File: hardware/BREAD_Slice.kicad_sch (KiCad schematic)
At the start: 27 parts, among them J1 I2C_01x04, J2 Conn_01x10_Female, J3 Screw_Terminal_01x02, J4 Screw_Terminal_01x02, J5 Screw_Terminal_01x02, J6 Screw_Terminal_01x02, J7 Screw_Terminal_01x02, J8 Screw_Terminal_01x02, Q1 TIP120, Q2 TIP120, Q3 TIP120, Q4 TIP120

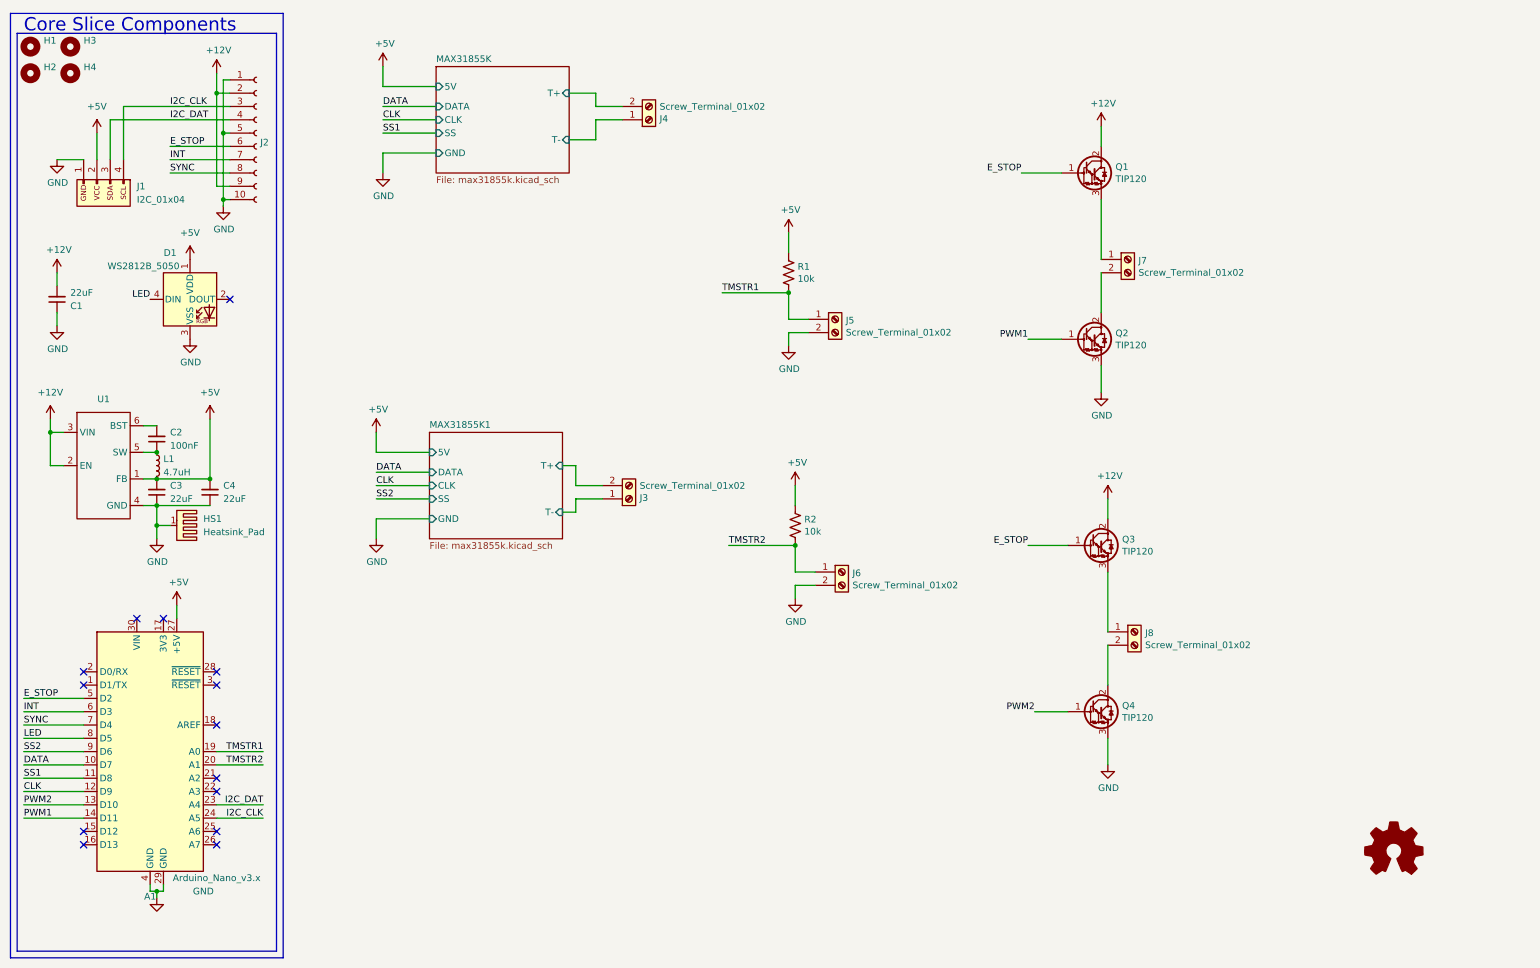
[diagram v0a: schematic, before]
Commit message: JLCPCB order rev-A
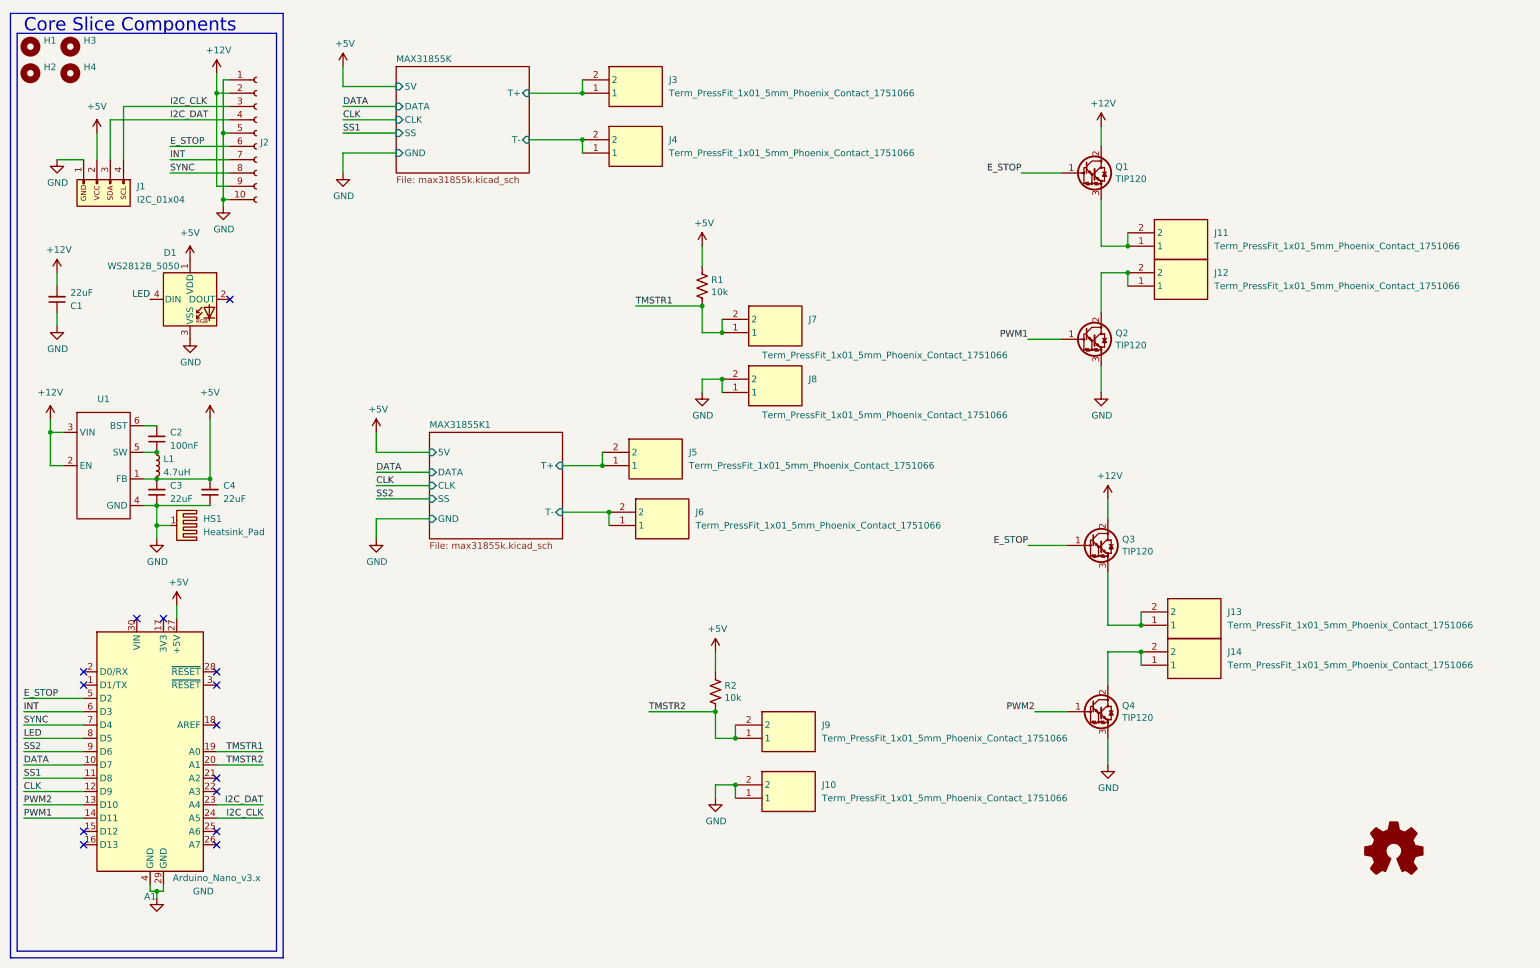
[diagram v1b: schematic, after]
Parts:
- removed J3, J4, J5, J6: Screw_Terminal_01x02, TerminalBlock_Phoenix:TerminalBlock_Phoenix_MPT-0,5-2-2.54_1x02_P2.54mm_Horizontal, symbol Connector:Screw_Terminal_01x02
- removed J7, J8: Screw_Terminal_01x02, TerminalBlock_Phoenix:TerminalBlock_Phoenix_MKDS-1,5-2_1x02_P5.00mm_Horizontal, symbol Connector:Screw_Terminal_01x02
- added J10, J11, J12, J13, J14, J3, J4, J5, J6, J7, J8, J9: Term_PressFit_1x01_5mm_Phoenix_Contact_1751066, 1751066, symbol kml-custom:Term_PressFit_1x01_5mm_Phoenix_Contact_1751066
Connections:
- net GND: now also J10.1, J10.2, J8.1, J8.2
- net MAX31855K/T+: now also J3.1, J3.2
- net MAX31855K/T-: now also J4.1, J4.2
- net MAX31855K1/T+: now also J5.1, J5.2
- net MAX31855K1/T-: now also J6.1, J6.2
- net TMSTR1: now also J7.1, J7.2
- net TMSTR2: now also J9.1, J9.2
- net at Q1.3 (E): now also J11.1, J11.2
- net at Q2.2 (C): now also J12.1, J12.2
- net at Q3.3 (E): now also J13.1, J13.2
- net at Q4.2 (C): now also J14.1, J14.2
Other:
- moved on the sheet: R1, R2
